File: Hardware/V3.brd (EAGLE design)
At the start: 100 x 80 mm, 21 parts

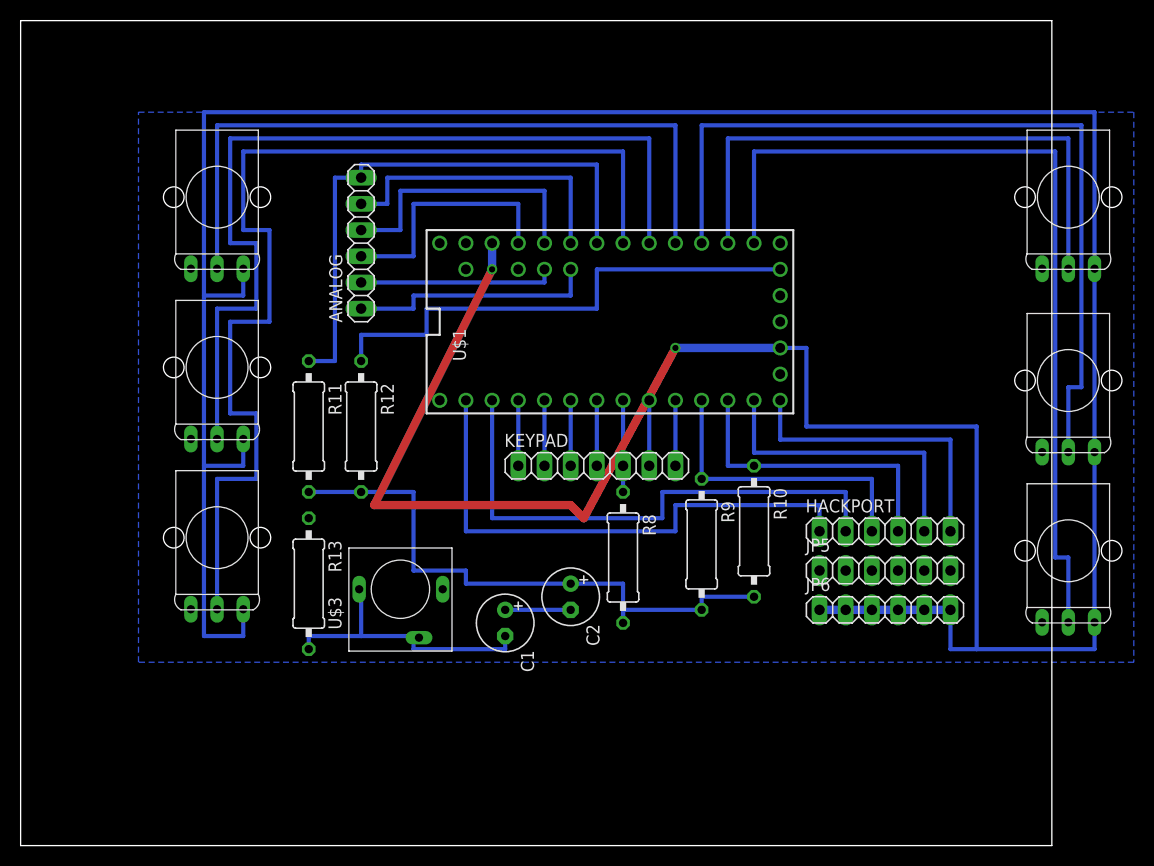
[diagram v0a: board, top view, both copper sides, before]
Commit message: New Example / New hardware version
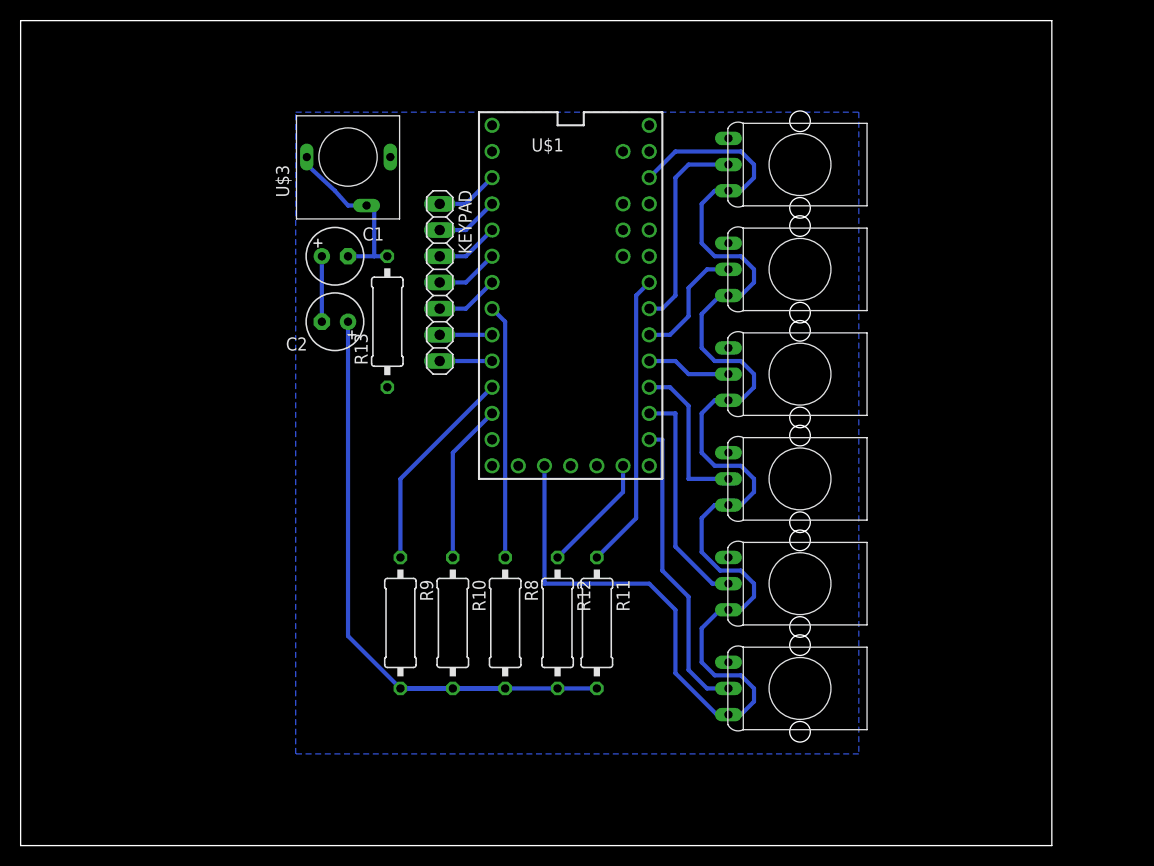
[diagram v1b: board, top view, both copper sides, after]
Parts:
- removed ANALOG, HACKPORT, JP5, JP6: (no value), pinhead:1X06
- moved R6 65.7 mm to (68.6, 66.0), turned to 270 degrees
- moved R5 52.2 mm to (68.6, 55.9), turned to 270 degrees
- moved R4 50.6 mm to (68.6, 45.7), turned to 270 degrees
- moved R2 44.9 mm to (68.6, 25.4), turned to 270 degrees
- moved U$3 42.2 mm to (31.8, 64.8)
- moved C1 39.2 mm to (30.5, 57.1), turned to 0 degrees
- moved C2 35.1 mm to (30.5, 50.8), turned to 180 degrees
- moved R11 33.8 mm to (55.9, 21.6)
- moved R1 33.6 mm to (68.6, 15.2), turned to 270 degrees
- moved R3 33.1 mm to (68.6, 35.6), turned to 270 degrees
- moved R10 30.5 mm to (41.9, 21.6)
- moved R9 30.2 mm to (36.8, 21.6)
- moved R12 26.9 mm to (52.1, 21.6)
- moved R13 26.5 mm to (35.6, 50.8), turned to 90 degrees
- moved KEYPAD 23.4 mm to (40.6, 54.6), turned to 270 degrees
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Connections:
- removed net N$17: ANALOG.2, U$1.A10
- removed net N$18: ANALOG.3, U$1.23/A9
- removed net N$19: ANALOG.4, U$1.22/A8
- removed net N$20: HACKPORT.1, U$1.0
- removed net N$21: HACKPORT.2, U$1.1
- removed net N$24: HACKPORT.5, U$1.11
- removed net N$25: HACKPORT.6, U$1.12
- removed net N$28: ANALOG.5, U$1.21/A7
- net GND: no longer JP5.1, JP5.2, JP5.3, JP5.4, JP5.5, JP5.6
- net N$10: now also KEYPAD.4, U$1.4; no longer KEYPAD.2, U$1.3
- net N$11: now also U$1.3; no longer U$1.4
- net N$12: now also KEYPAD.2, U$1.2; no longer KEYPAD.4, U$1.5
- net N$13: no longer KEYPAD.5
- net N$16: now also KEYPAD.1, U$1.1; no longer ANALOG.1, U$1.A11
- net N$22: no longer HACKPORT.3
- net N$23: no longer HACKPORT.4
- net N$29: no longer ANALOG.6
- net N$7: now also KEYPAD.5, U$1.5; no longer KEYPAD.1, U$1.2
- net N$8: no longer JP6.1, JP6.2, JP6.3, JP6.4, JP6.5, JP6.6
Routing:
- net N$8: track 365.1 -> 139.9 mm, vias 2 -> 0
- net N$6: track 102.8 -> 20.2 mm
- net N$5: track 86.4 -> 11.9 mm
- net N$3: track 81.2 -> 15.5 mm
- net N$4: track 69.8 -> 8.21 mm
- net N$1: track 85.0 -> 29.3 mm
- net N$20: track 52.1 -> 0.00 mm
- net N$21: track 52.1 -> 0.00 mm
- net N$26: track 49.5 -> 11.5 mm
- net N$2: track 55.8 -> 22.1 mm
- net N$25: track 29.2 -> 0.00 mm
- net N$28: track 29.2 -> 0.00 mm
- net N$24: track 29.2 -> 0.00 mm
- net N$19: track 26.7 -> 0.00 mm
- net N$29: track 54.6 -> 28.8 mm
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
